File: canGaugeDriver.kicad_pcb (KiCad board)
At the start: 2 copper layers, 80 x 41.4 mm, 50 parts, among them J1 CANbed 1.0 Interface, J2 348260240, U1 TPL7407LA, U2 TPL7407LA

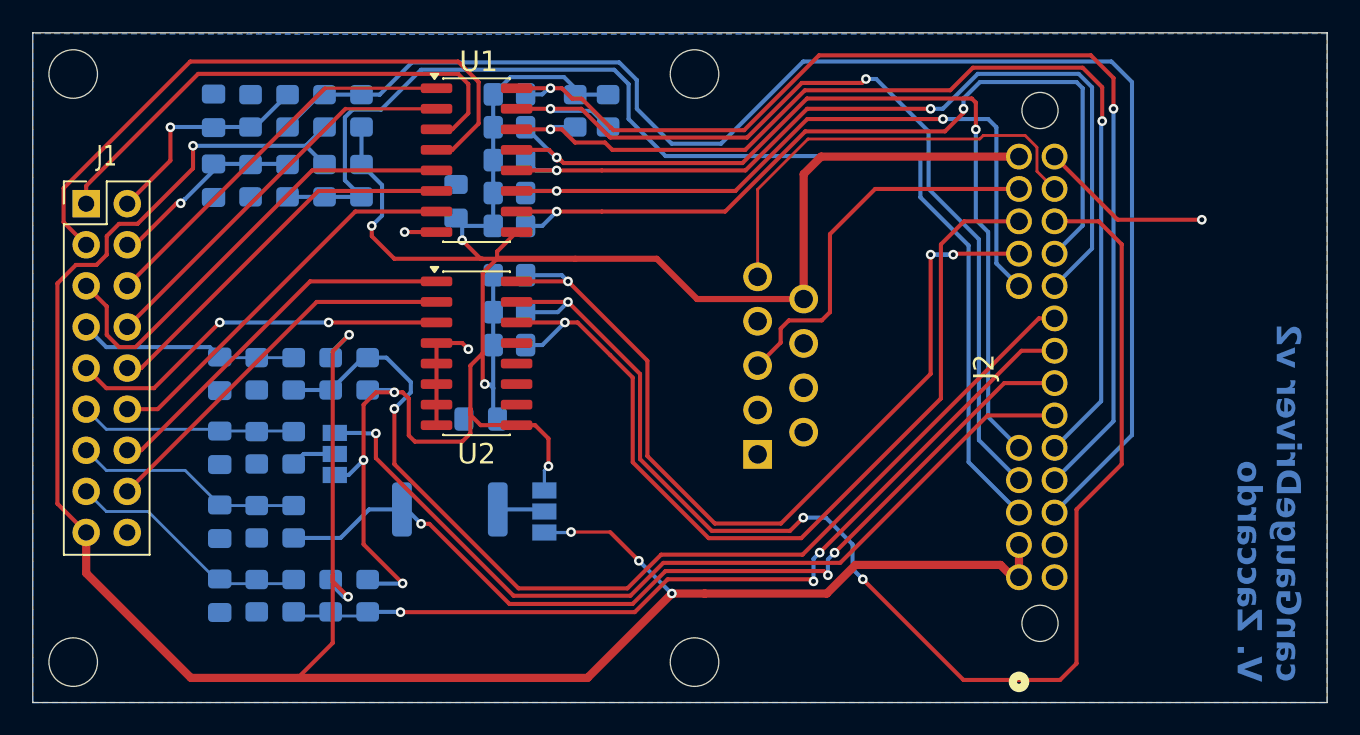
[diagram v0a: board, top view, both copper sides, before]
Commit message: minor cleanup
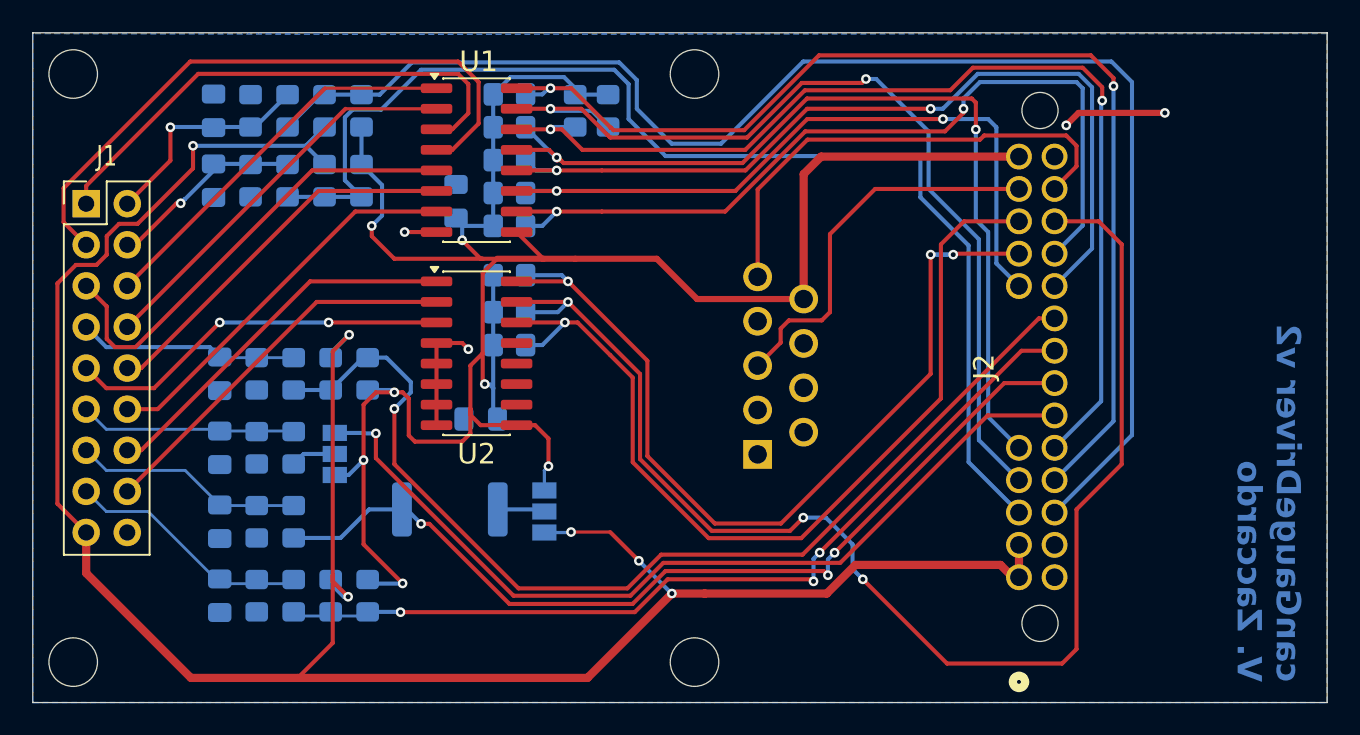
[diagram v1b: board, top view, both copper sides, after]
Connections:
- net /AI0 renamed /A0_IN
- net /AI1 renamed /A1_IN
- net /AI2 renamed /A2_IN
- net /AI3 renamed /A3_IN
- net /D0_RX renamed /D0
- net /D10_OIL renamed /D10
- net /D11_TACH renamed /D11
- net /D12_ALT renamed /D12
- net /D1_TX renamed /D1
- net /D2_SRS renamed /D2
- net /D3_SPEED renamed /D3
- net /D4_CEL renamed /D4
- net /D5_COOL renamed /D5
- net /D6_ABS renamed /D6
- net /D8_SEATBELT renamed /D8
- net /D9_FUEL renamed /D9
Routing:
- net GND: track 19.9 -> 15.6 mm, vias 3 -> 4
- net /CANL: track 27.4 -> 30.0 mm
- net /D11_OUT: track 84.1 -> 82.7 mm
